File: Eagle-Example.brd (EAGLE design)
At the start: 50 x 50 mm, 1 part

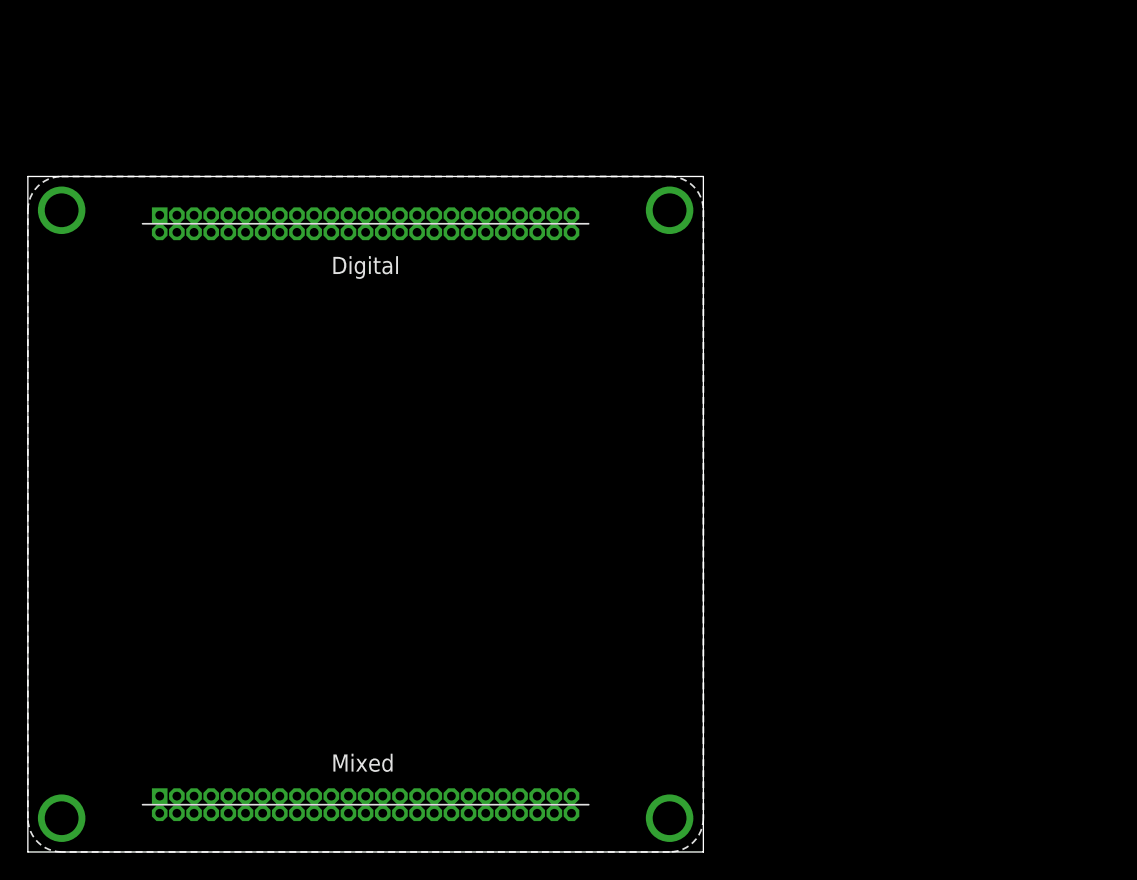
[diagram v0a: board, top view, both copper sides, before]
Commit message: Started BlackEdge Nxt branch
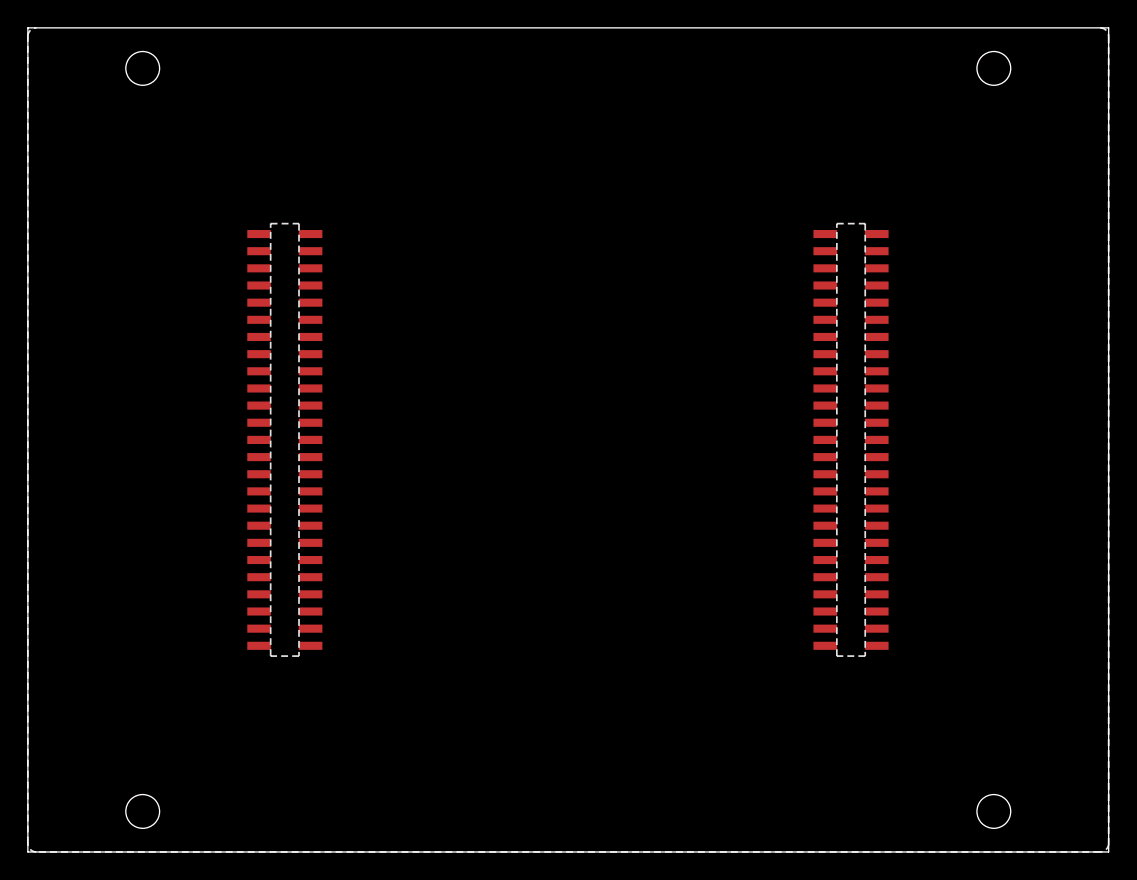
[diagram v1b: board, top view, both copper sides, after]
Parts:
- removed U$1: BE-CARRIER, BlackEdge:BE-CARRIER
- added T1: (no value), amino:MEZZANINE
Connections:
- new net +3V3: T1.E47
- new net +5V: T1.E22
- new net +VE0: T1.E26
- new net +VE1: T1.E27
- new net +VE2: T1.E28
- new net +VE3: T1.E23
- new net +VE4: T1.E24
- new net +VE5: T1.E25
- new net +VW0: T1.W26
- new net +VW2: T1.W28
- new net +VW3: T1.W29
- new net +VW4: T1.W22
- new net +VW5: T1.W23
- new net +VW6: T1.W24
- new net +VW7: T1.W25
- new net GND0: T1.E1
- new net GND1: T1.E2
- new net GND10: T1.W47
- new net GND11: T1.W48
- new net GND12: T1.W49
- new net GND13: T1.W50
- new net GND2: T1.E3
- new net GND3: T1.E48
- new net GND4: T1.E49
- new net GND5: T1.E50
- new net GND6: T1.W1
- new net GND7: T1.W2
- new net GND8: T1.W3
- new net GND9: T1.W4
- new net VCC: T1.E4
- new net VPP: T1.E29
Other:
- board size 50 x 50 mm -> 80 x 61 mm
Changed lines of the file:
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@@
 <?xml version="1.0" encoding="utf-8"?>
 <!DOCTYPE eagle SYSTEM "eagle.dtd">
-<eagle version="7.7.0">
+<eagle version="7.5.0">
 <drawing>
 <settings>
-<setting alwaysvectorfont="no"/>
+<setting alwaysvectorfont="yes"/>
 <setting verticaltext="up"/>
 </settings>
-<grid distance="0.05" unitdist="inch" unit="mm" style="lines" multiple="1" display="no" altdistance="0.025" altunitdist="inch" altunit="mm"/>
+<grid distance="1" unitdist="mm" unit="mm" style="lines" multiple="1" display="no" altdistance="0.025" altunitdist="inch" altunit="mil"/>
 <layers>
-<layer number="1" name="Top" color="4" fill="1" visible="yes" active="yes"/>
+<layer number="1" name="Top" color="30" fill="1" visible="yes" active="yes"/>
 <layer number="2" name="Route2" color="1" fill="3" visible="no" active="no"/>
 <layer number="3" name="Route3" color="4" fill="3" visible="no" active="no"/>
 <layer number="14" name="Route14" color="1" fill="6" visible="no" active="no"/>
 <layer number="15" name="Route15" color="4" fill="6" visible="no" active="no"/>
-<layer number="16" name="Bottom" color="1" fill="1" visible="yes" active="yes"/>
+<layer number="16" name="Bottom" color="46" fill="1" visible="yes" active="yes"/>
 <layer number="17" name="Pads" color="2" fill="1" visible="yes" active="yes"/>
 <layer number="18" name="Vias" color="2" fill="1" visible="yes" active="yes"/>
@@
 <layer number="56" name="wert" color="7" fill="1" visible="no" active="no"/>
 <layer number="57" name="tCAD" color="7" fill="1" visible="no" active="no"/>
+<layer number="58" name="bCAD" color="7" fill="1" visible="no" active="no"/>
 <layer number="59" name="tCarbon" color="7" fill="1" visible="no" active="no"/>
 <layer number="60" name="bCarbon" color="7" fill="1" visible="no" active="no"/>
@@
 <layer number="89" name="SimProbes" color="9" fill="1" visible="yes" active="yes"/>
 <layer number="90" name="Modules" color="5" fill="1" visible="no" active="no"/>
-<layer number="91" name="Nets" color="2" fill="1" visible="no" active="no"/>
+<layer number="91" name="Nets" color="30" fill="1" visible="no" active="no"/>
 <layer number="92" name="Busses" color="1" fill="1" visible="no" active="no"/>
 <layer number="93" name="Pins" color="2" fill="1" visible="no" active="no"/>
-<layer number="94" name="Symbols" color="4" fill="1" visible="no" active="no"/>
+<layer number="94" name="Symbols" color="31" fill="1" visible="no" active="no"/>
 <layer number="95" name="Names" color="7" fill="1" visible="no" active="no"/>
 <layer number="96" name="Values" color="7" fill="1" visible="no" active="no"/>
@@
 <layer number="115" name="ReferenceISLANDS" color="7" fill="1" visible="yes" active="yes"/>
 <layer number="116" name="Patch_BOT" color="9" fill="4" visible="yes" active="yes"/>
+<layer number="117" name="PM_Ref" color="26" fill="1" visible="no" active="no"/>
 <layer number="118" name="Rect_Pads" color="7" fill="1" visible="yes" active="yes"/>
+<layer number="119" name="PF_Ref" color="31" fill="1" visible="no" active="no"/>
+<layer number="120" name="WFL_Ref" color="25" fill="1" visible="no" active="no"/>
 <layer number="121" name="_tsilk" color="7" fill="1" visible="yes" active="yes"/>
 <layer number="122" name="_bsilk" color="7" fill="1" visible="yes" active="yes"/>
@@
 <layer number="128" name="_bValues" color="7" fill="1" visible="yes" active="yes"/>
 <layer number="129" name="Mask" color="7" fill="1" visible="yes" active="yes"/>
+<layer number="130" name="SMDSTROOK" color="7" fill="1" visible="no" active="no"/>
 <layer number="131" name="tAdjust" color="7" fill="1" visible="yes" active="yes"/>
 <layer number="132" name="bAdjust" color="7" fill="1" visible="yes" active="yes"/>
+<layer number="133" name="bottom_silk" color="7" fill="1" visible="no" active="no"/>
+<layer number="134" name="silk_top" color="7" fill="1" visible="no" active="no"/>
+<layer number="135" name="silk_bottom" color="7" fill="1" visible="no" active="no"/>
+<layer number="136" name="silktop" color="7" fill="1" visible="no" active="no"/>
+<layer number="137" name="silkbottom" color="7" fill="1" visible="no" active="no"/>
+<layer number="138" name="EEE" color="7" fill="1" visible="no" active="no"/>
+<layer number="139" name="_tKeepout" color="7" fill="1" visible="no" active="no"/>
+<layer number="140" name="mbKeepout" color="7" fill="1" visible="no" active="no"/>
+<layer number="141" name="ASSEMBLY_TOP" color="7" fill="1" visible="no" active="no"/>
+<layer number="142" name="mbRestrict" color="7" fill="1" visible="no" active="no"/>
+<layer number="143" name="PLACE_BOUND_TOP" color="7" fill="1" visible="no" active="no"/>
 <layer number="144" name="Drill_legend" color="7" fill="1" visible="yes" active="yes"/>
+<layer number="145" name="DrillLegend_01-16" color="7" fill="1" visible="no" active="no"/>
+<layer number="146" name="DrillLegend_01-20" color="7" fill="1" visible="no" active="no"/>
+<layer number="147" name="PIN_NUMBER" color="7" fill="1" visible="no" active="no"/>
+<layer number="148" name="DrillLegend_01-20" color="7" fill="1" visible="no" active="no"/>
+<layer number="149" name="DrillLegend_02-15" color="7" fill="1" visible="no" active="no"/>
 <layer number="150" name="Notes" color="7" fill="1" visible="yes" active="yes"/>
 <layer number="151" name="HeatSink" color="14" fill="1" visible="yes" active="yes"/>
@@
 <layer number="154" name="FabDoc2" color="7" fill="1" visible="yes" active="yes"/>
 <layer number="155" name="FabDoc3" color="7" fill="1" visible="yes" active="yes"/>
+<layer number="166" name="AntennaArea" color="7" fill="1" visible="no" active="no"/>
+<layer number="168" name="4mmHeightArea" color="7" fill="1" visible="no" active="no"/>
+<layer number="191" name="mNets" color="7" fill="1" visible="no" active="no"/>
+<layer number="192" name="mBusses" color="7" fill="1" visible="no" active="no"/>
+<layer number="193" name="mPins" color="7" fill="1" visible="no" active="no"/>
+<layer number="194" name="mSymbols" color="7" fill="1" visible="no" active="no"/>
+<layer number="195" name="mNames" color="7" fill="1" visible="no" active="no"/>
+<layer number="196" name="mValues" color="7" fill="1" visible="no" active="no"/>
 <layer number="199" name="Contour" color="7" fill="1" visible="yes" active="yes"/>
 <layer number="200" name="200bmp" color="1" fill="10" visible="no" active="no"/>
@@
 <layer number="250" name="Descript" color="3" fill="1" visible="no" active="no"/>
 <layer number="251" name="SMDround" color="12" fill="11" visible="no" active="no"/>
+<layer number="253" name="Extra" color="7" fill="1" visible="no" active="no"/>
 <layer number="254" name="OrgLBR" color="13" fill="1" visible="yes" active="yes"/>
 <layer number="255" name="routoute" color="7" fill="1" visible="yes" active="yes"/>
@@
 <board>
 <plain>
-<wire x1="0" y1="0" x2="50" y2="0" width="0" layer="20"/>
-<wire x1="50" y1="0" x2="50" y2="50" width="0" layer="20"/>
-<wire x1="50" y1="50" x2="0" y2="50" width="0" layer="20"/>
-<wire x1="0" y1="50" x2="0" y2="0" width="0" layer="20"/>
-<dimension x1="50" y1="50" x2="0" y2="50" x3="25" y3="57.15" textsize="1.778" layer="21"/>
-<dimension x1="0" y1="50" x2="0" y2="0" x3="-7.62" y3="25" textsize="1.778" layer="21"/>
+<wire x1="0" y1="0" x2="80" y2="0" width="0" layer="20"/>
+<wire x1="80" y1="0" x2="80" y2="61" width="0" layer="20"/>
+<wire x1="80" y1="61" x2="0" y2="61" width="0" layer="20"/>
+<wire x1="0" y1="61" x2="0" y2="0" width="0" layer="20"/>
 </plain>
 <attributes>
@@
 </autorouter>
 <elements>
-<element name="U$1" library="BlackEdge" package="BE-CARRIER" value="BE-CARRIER" x="25" y="25"/>
+<element name="T1" library="amino" package="MEZZANINE" value="" x="40" y="30.5"/>
 </elements>
 <signals>
+<signal name="GND0">
+<contactref element="T1" pad="E1"/>
+</signal>
+<signal name="GND1">
+<contactref element="T1" pad="E2"/>
+</signal>
+<signal name="GND2">
+<contactref element="T1" pad="E3"/>
+</signal>
+<signal name="VCC">
+<contactref element="T1" pad="E4"/>
+</signal>
+<signal name="+5V">
+<contactref element="T1" pad="E22"/>
+</signal>
+<signal name="+VE3">
+<contactref element="T1" pad="E23"/>
+</signal>
+<signal name="+VE4">
+<contactref element="T1" pad="E24"/>
+</signal>
+<signal name="+VE5">
+<contactref element="T1" pad="E25"/>
+</signal>
+<signal name="+VE0">
+<contactref element="T1" pad="E26"/>
+</signal>
+<signal name="+VE1">
+<contactref element="T1" pad="E27"/>
+</signal>
+<signal name="+VE2">
+<contactref element="T1" pad="E28"/>
+</signal>
+<signal name="VPP">
+<contactref element="T1" pad="E29"/>
+</signal>
+<signal name="+3V3">
+<contactref element="T1" pad="E47"/>
+</signal>
+<signal name="GND3">
+<contactref element="T1" pad="E48"/>
+</signal>
+<signal name="GND4">
+<contactref element="T1" pad="E49"/>
+</signal>
+<signal name="GND5">
+<contactref element="T1" pad="E50"/>
+</signal>
+<signal name="GND6">
+<contactref element="T1" pad="W1"/>
+</signal>
+<signal name="GND7">
+<contactref element="T1" pad="W2"/>
+</signal>
+<signal name="GND8">
+<contactref element="T1" pad="W3"/>
+</signal>
+<signal name="GND9">
+<contactref element="T1" pad="W4"/>
+</signal>
+<signal name="+VW4">
+<contactref element="T1" pad="W22"/>
+</signal>
+<signal name="+VW5">
+<contactref element="T1" pad="W23"/>
+</signal>
+<signal name="+VW6">
+<contactref element="T1" pad="W24"/>
+</signal>
+<signal name="+VW7">
+<contactref element="T1" pad="W25"/>
+</signal>
+<signal name="+VW0">
+<contactref element="T1" pad="W26"/>
+</signal>
+<signal name="+VW2">
+<contactref element="T1" pad="W28"/>
+</signal>
+<signal name="+VW3">
+<contactref element="T1" pad="W29"/>
+</signal>
+<signal name="GND10">
+<contactref element="T1" pad="W47"/>
+</signal>
+<signal name="GND11">
+<contactref element="T1" pad="W48"/>
+</signal>
+<signal name="GND12">
+<contactref element="T1" pad="W49"/>
+</signal>
+<signal name="GND13">
+<contactref element="T1" pad="W50"/>
+</signal>
 </signals>
 </board>
